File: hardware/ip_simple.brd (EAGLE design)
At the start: 28 x 31 mm, 32 parts, among them Q4 irml9301, Q7 irml9301, T1 BC846, T3 BC846, Y1 32768Hz CFPX-217 12.5pF

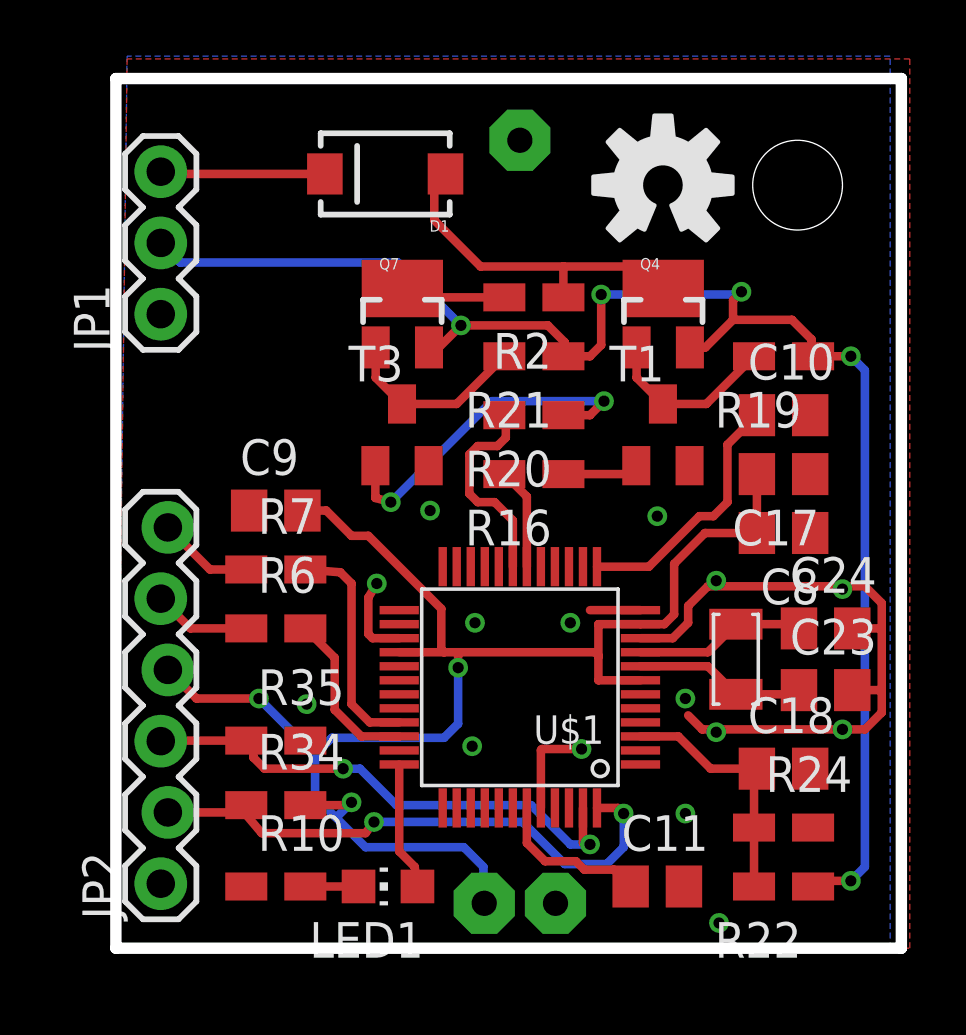
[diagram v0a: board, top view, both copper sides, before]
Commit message: sent to manufacturer
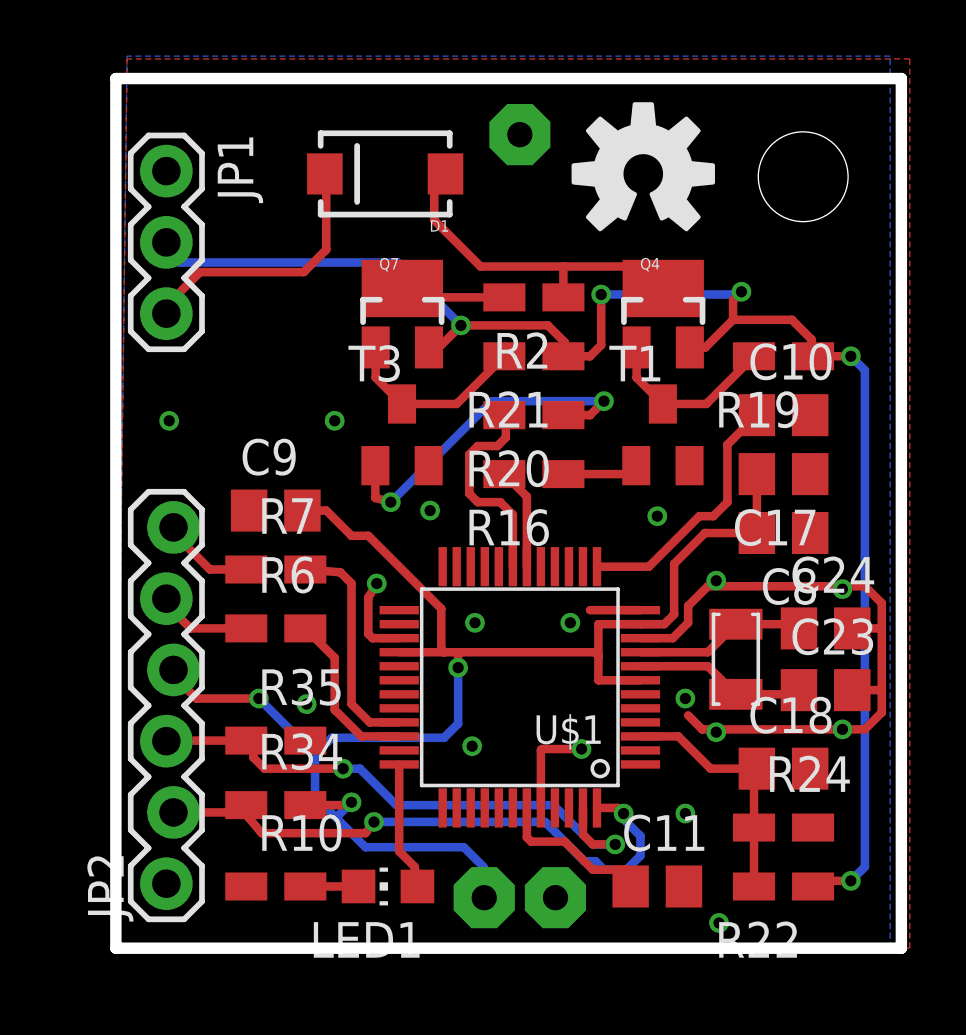
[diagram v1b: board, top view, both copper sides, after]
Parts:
- moved JP1 5.10 mm to (1.80, 27.7), turned to 270 degrees
- moved U$7 0.81 mm to (18.8, 27.6)
- moved G1 0.20 mm to (14.4, 15.4)
- moved JP2 0.20 mm to (1.80, 2.30)
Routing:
- net AVP: track 5.88 -> 9.55 mm
- net TEST: track 18.7 -> 20.1 mm
- net RST: track 20.3 -> 21.3 mm
- net GND: vias 15 -> 17
